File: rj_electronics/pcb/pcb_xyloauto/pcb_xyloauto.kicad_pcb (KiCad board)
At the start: 2 copper layers, 200 x 37 mm, 21 parts, among them J1 Screw_Terminal_01x08, J3 Conn_01x02_Pin, J4 Barrel_Jack, J5 Screw_Terminal_01x08, U1 Sparkfun_Pro_Micro, U2 ULN2803A, U4 LM317_TO-220

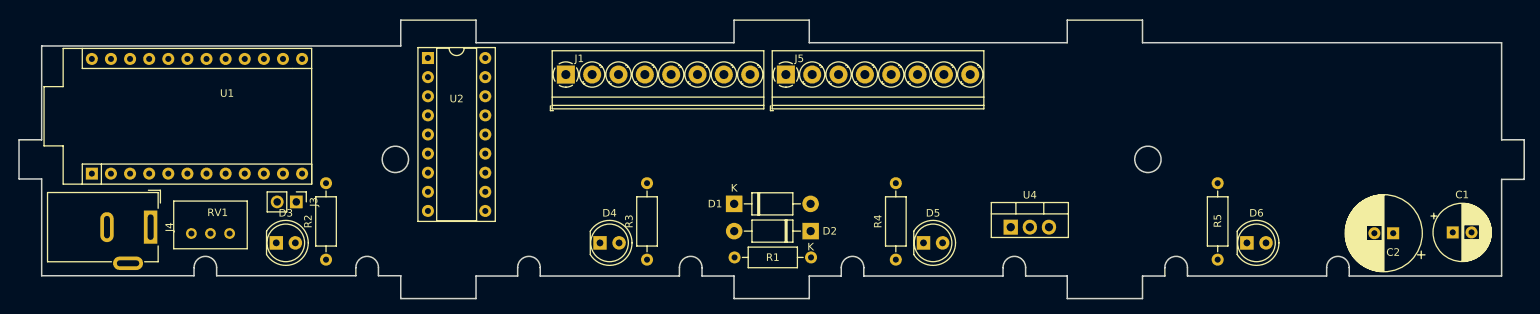
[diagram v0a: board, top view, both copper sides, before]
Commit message: nc
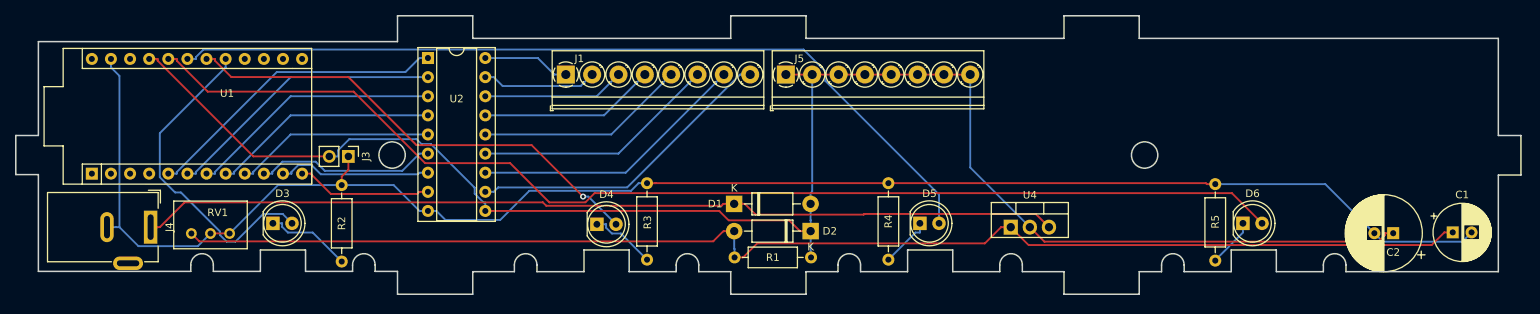
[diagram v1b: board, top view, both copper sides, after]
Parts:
- moved J3 9.19 mm to (74.5, 127.8)
- moved D6 2.65 mm to (193.4, 136.7)
- moved D5 2.64 mm to (150.5, 136.7)
- moved D3 2.64 mm to (64.5, 136.7)
- moved D4 2.51 mm to (107.6, 136.8)
- moved R2 2.10 mm to (73.7, 141.7)
- moved R4 0.99 mm to (146.3, 141.5)
- moved R5 0.34 mm to (189.7, 141.6)
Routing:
- net VOUT: track 0.00 -> 223.2 mm
- net GND: track 0.00 -> 220.4 mm
- net Net-(D2-A): track 0.00 -> 175.4 mm
- net LED4: track 0.00 -> 155.5 mm
- net VIN: track 0.00 -> 122.4 mm
- net LED3: track 0.00 -> 113.1 mm
- net LED2: track 0.00 -> 63.7 mm, vias 0 -> 1
- net LED1: track 0.00 -> 42.8 mm
- net Net-(J1-Pin_8): track 0.00 -> 41.7 mm
- net Net-(U1-D2): track 0.00 -> 41.0 mm
- net Net-(U1-~D3): track 0.00 -> 37.4 mm
- net Net-(J1-Pin_7): track 0.00 -> 37.1 mm
- net Net-(U1-D4/A6): track 0.00 -> 33.8 mm
- net Net-(J1-Pin_6): track 0.00 -> 32.6 mm
- net Net-(U1-~D5): track 0.00 -> 30.2 mm
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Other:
- outline, holes or cut-outs redrawn
